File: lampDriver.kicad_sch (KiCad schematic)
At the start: 61 parts, among them IC8 FAN3100TSX, Q4 BC807, T4 IMBG120R181M2HXTMA1, U1 OPA2356AIDGKR, U3 LM2902

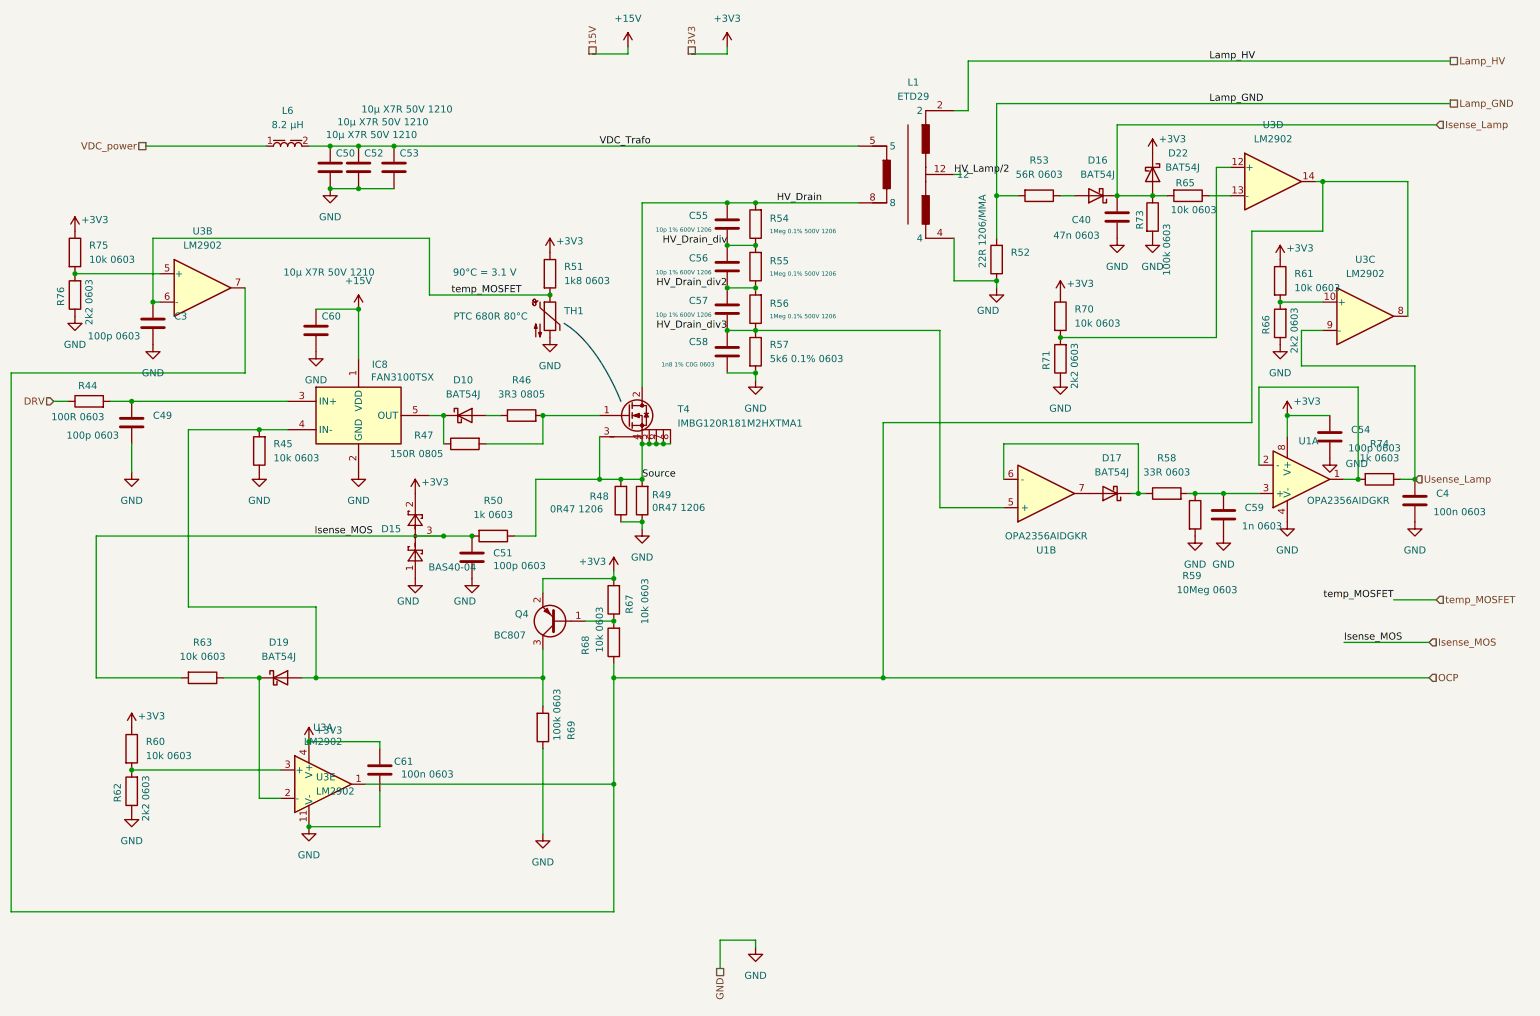
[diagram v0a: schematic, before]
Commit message: V2 PCB
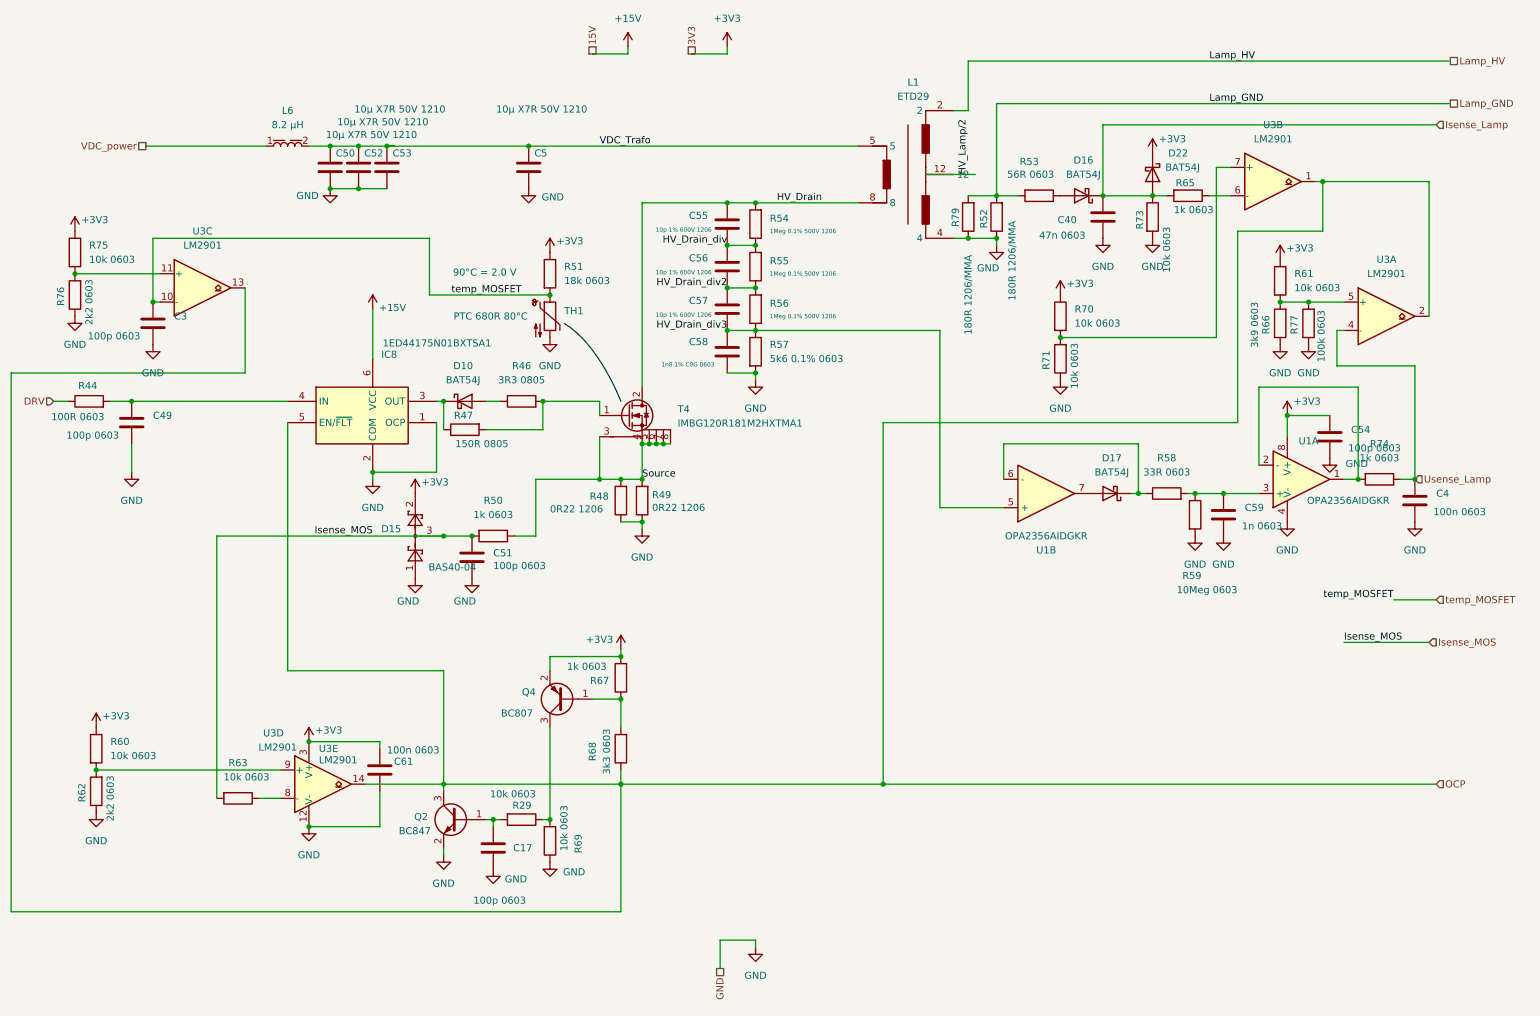
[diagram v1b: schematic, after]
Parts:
- removed C60: 10µ X7R 50V 1210, Capacitor_SMD:C_1210_3225Metric, symbol Device:C
- removed D19: BAT54J, Diode_SMD:D_SOD-323F, symbol Diode:BAT54J
- removed IC8: FAN3100TSX, SOT95P280X145-5N, symbol Hansmann:FAN3100TSX
- removed R45: 10k 0603, Resistor_SMD:R_0603_1608Metric, symbol Device:R
- removed U3: LM2902, Package_SO:TSSOP-14_4.4x5mm_P0.65mm, symbol Amplifier_Operational:LM2902
- added C17: 100p 0603, Capacitor_SMD:C_0603_1608Metric, symbol Device:C
- added C5: 10µ X7R 50V 1210, Capacitor_SMD:C_1210_3225Metric, symbol Device:C
- added IC8: 1ED44175N01BXTSA1, SOT95P280X145-6N, symbol Hansmann:1ED44175N01BXTSA1
- added Q2: BC847, Package_TO_SOT_SMD:SOT-23, symbol Transistor_BJT:BC847
- added R29: 10k 0603, Resistor_SMD:R_0603_1608Metric, symbol Device:R
- added R77: 100k 0603, Resistor_SMD:R_0603_1608Metric, symbol Device:R
- added R79: 180R 1206/MMA, Resistor_SMD:R_1206_3216Metric, symbol Device:R
- added U3: LM2901, Package_SO:TSSOP-14_4.4x5mm_P0.65mm, symbol Comparator:LM2901
- R48, R49: value 0R47 1206 -> 0R22 1206
- R51: value 1k8 0603 -> 18k 0603
- R52: value 22R 1206/MMA -> 180R 1206/MMA
- R65, R67: value 10k 0603 -> 1k 0603
- R66: value 2k2 0603 -> 3k9 0603
- R68: value 10k 0603 -> 3k3 0603
- R69, R73: value 100k 0603 -> 10k 0603
- R71: value 2k2 0603 -> 10k 0603
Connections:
- net +15V: now also IC8.6 (VCC)
- net +3V3: now also U3.3 (V+)
- net GND: now also C17.2, C5.2, IC8.1 (OCP), IC8.2 (COM), Q2.2 (E), R77.1, R79.1, U3.12 (V-)
- net HV_Lamp/2: now also L1.12
- net Lamp_GND: now also R79.2
- net OCP: now also IC8.5 (EN/~{FLT}), Q2.3 (C), U3.1, U3.13, U3.14, U3.2
- net Usense_Lamp: now also U3.4 (-)
- net VDC_Trafo: now also C5.1
- net temp_MOSFET: now also U3.10 (-)
- net at C49.1, R44.2: now also IC8.4 (IN)
- net at Q4.3 (C), R69.2: now also R29.1
- net at R61.2, R66.2: now also R77.2, U3.5 (+)
- net at R65.1: now also U3.6 (-)
- net at R75.2, R76.2: now also U3.11 (+)
- net at D10.1 (K), R47.1: now also IC8.3 (OUT)
- net at R60.2, R62.2: now also U3.9 (+)
- net at R70.2, R71.2: now also U3.7 (+)
- net at R63.1: now also U3.8 (-)
- new net: C17.1, Q2.1 (B), R29.2
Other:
- note added: "90°C = 2.0 V"
- note removed: "90°C = 3.1 V"
- moved on the sheet: C40, C53, D10, D16, Q4, R46, R47, R52, R60, R62, R63, R67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
